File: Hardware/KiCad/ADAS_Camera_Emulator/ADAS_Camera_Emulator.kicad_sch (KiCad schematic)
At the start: 0 parts

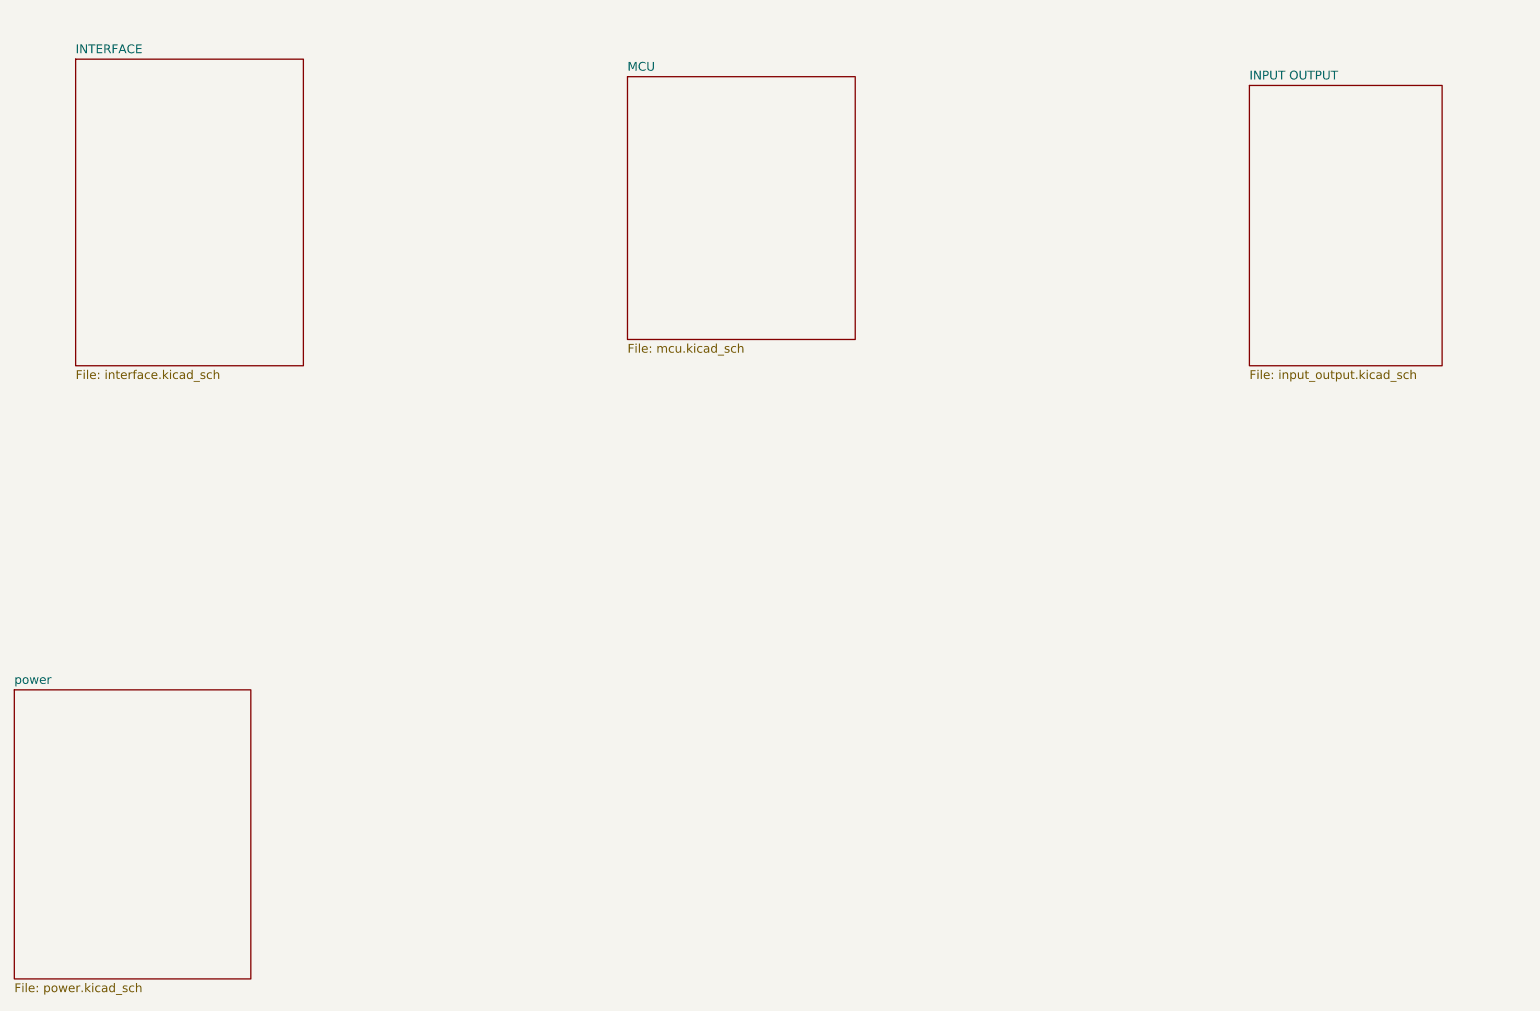
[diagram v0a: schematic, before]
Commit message: just shematic stuff
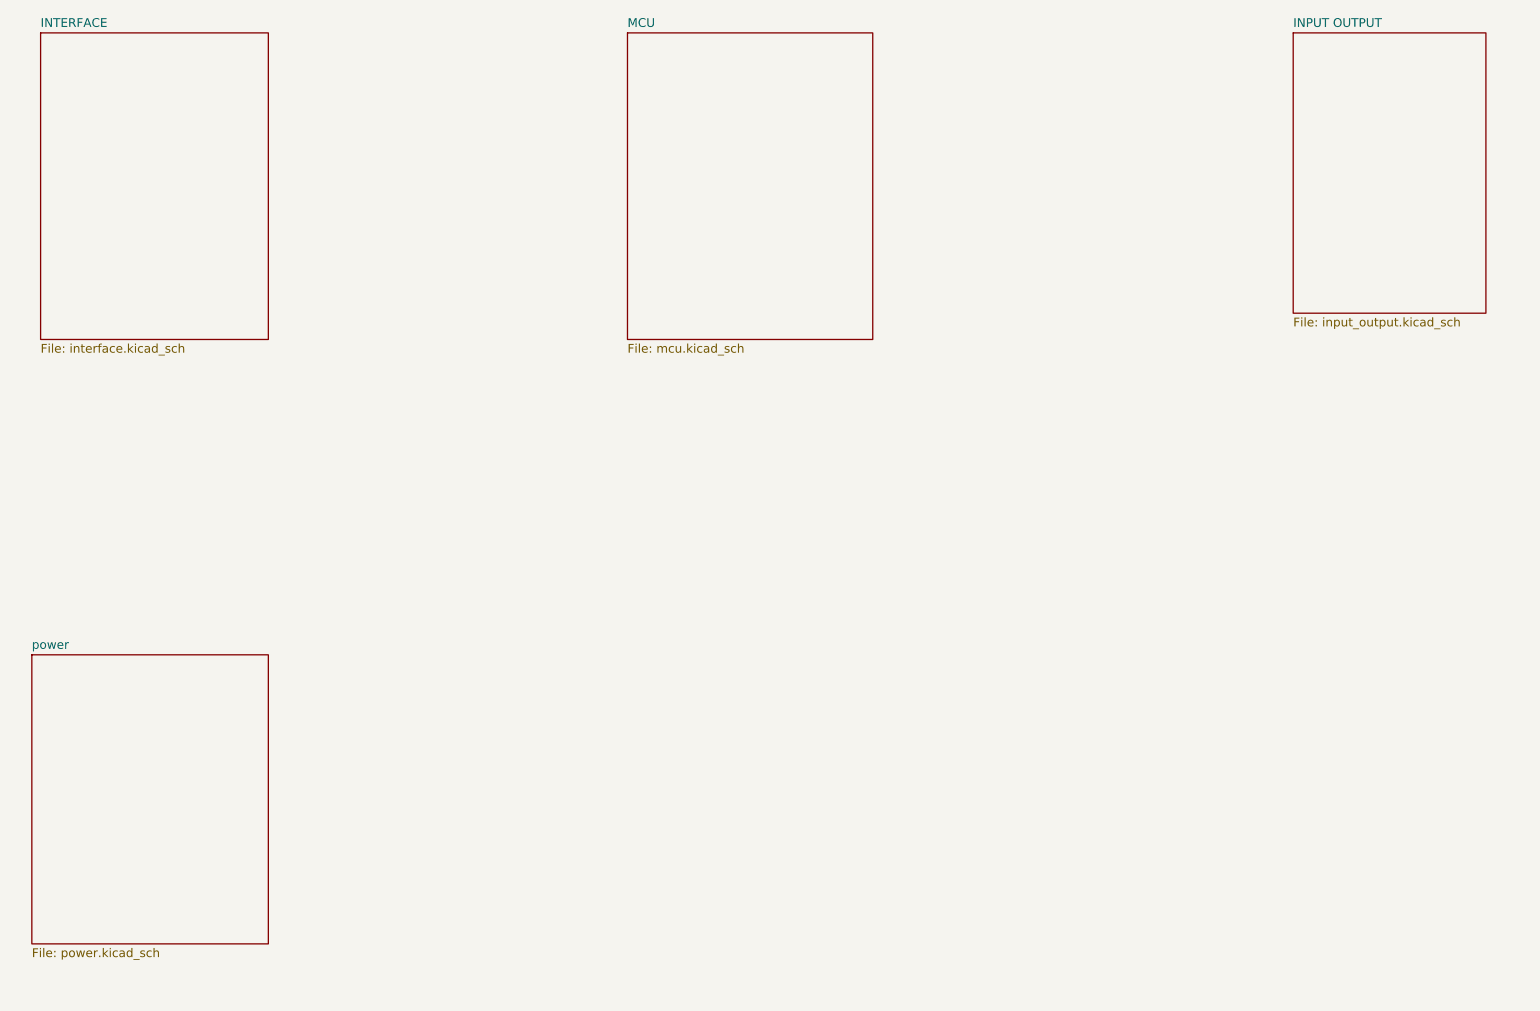
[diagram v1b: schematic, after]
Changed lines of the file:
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@@
 	)
 	(sheet
-		(at 212.09 49.53)
+		(at 218.44 41.91)
 		(size 27.94 40.64)
 		(exclude_from_sim no)
@@
 		)
 		(property "Sheetname" "INPUT OUTPUT"
-			(at 212.09 48.8184 0)
+			(at 218.44 41.1984 0)
 			(effects
 				(font
@@
 		)
 		(property "Sheetfile" "input_output.kicad_sch"
-			(at 212.09 90.7546 0)
+			(at 218.44 83.1346 0)
 			(effects
 				(font
@@
 	)
 	(sheet
-		(at 33.02 137.16)
+		(at 35.56 132.08)
 		(size 34.29 41.91)
 		(exclude_from_sim no)
@@
 			(width 0.1524)
 			(type solid)
+			(color 87 190 35 1)
 		)
 		(fill
-			(color 0 0 0 0.0000)
+			(color 87 190 35 1.0000)
 		)
 		(property "Sheetname" "power"
-			(at 33.02 136.4484 0)
+			(at 35.56 131.3684 0)
 			(effects
 				(font
@@
 		)
 		(property "Sheetfile" "power.kicad_sch"
-			(at 33.02 179.6546 0)
+			(at 35.56 174.5746 0)
 			(effects
 				(font
@@
 	)
 	(sheet
-		(at 121.92 48.26)
-		(size 33.02 38.1)
+		(at 121.92 41.91)
+		(size 35.56 44.45)
 		(exclude_from_sim no)
 		(in_bom yes)
@@
 		)
 		(property "Sheetname" "MCU"
-			(at 121.92 47.5484 0)
+			(at 121.92 41.1984 0)
 			(effects
 				(font
@@
 	)
 	(sheet
-		(at 41.91 45.72)
+		(at 36.83 41.91)
 		(size 33.02 44.45)
 		(exclude_from_sim no)
@@
 		)
 		(property "Sheetname" "INTERFACE"
-			(at 41.91 45.0084 0)
+			(at 36.83 41.1984 0)
 			(effects
 				(font
@@
 		)
 		(property "Sheetfile" "interface.kicad_sch"
-			(at 41.91 90.7546 0)
+			(at 36.83 86.9446 0)
 			(effects
 				(font
